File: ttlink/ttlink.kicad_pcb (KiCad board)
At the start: 2 copper layers, 38.6 x 17.9 mm, 10 parts, among them J1 USB, J2 TTL, U1 CH340G, Y1 12MHz

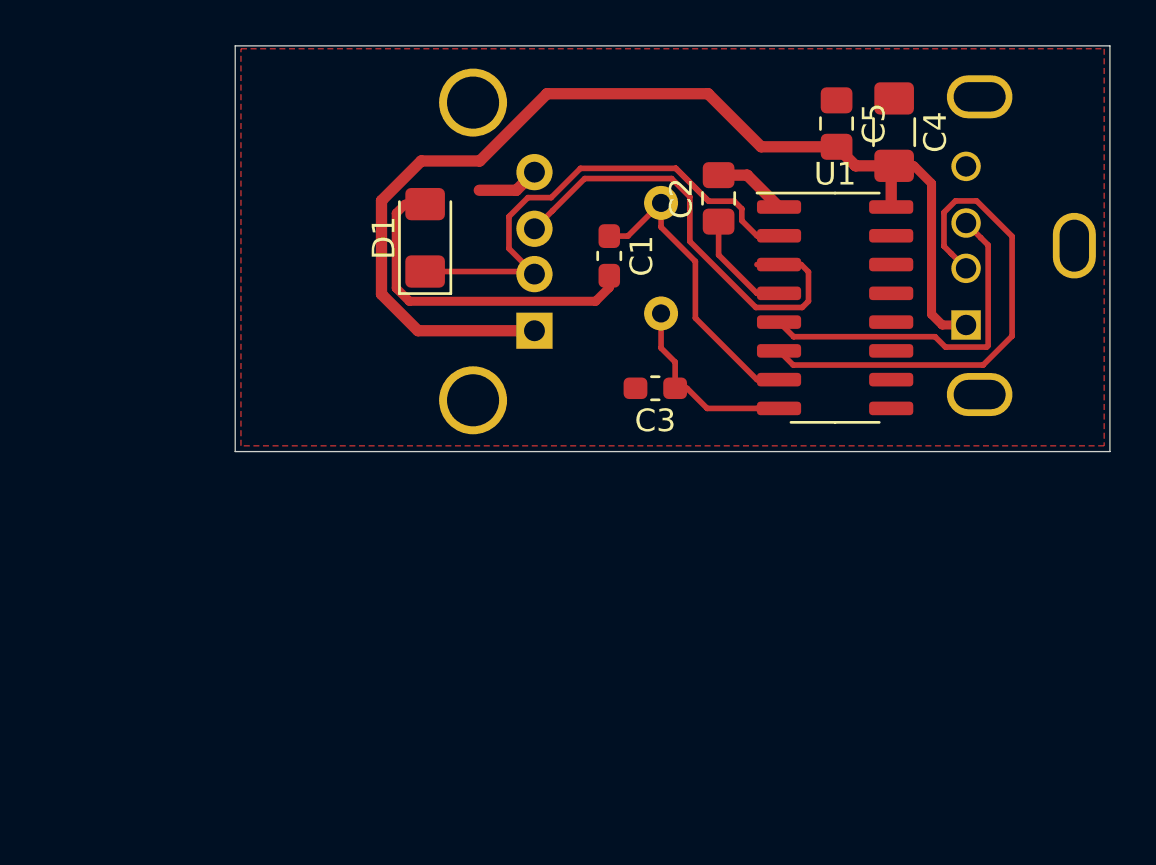
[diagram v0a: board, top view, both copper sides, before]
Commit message: PCB layed out
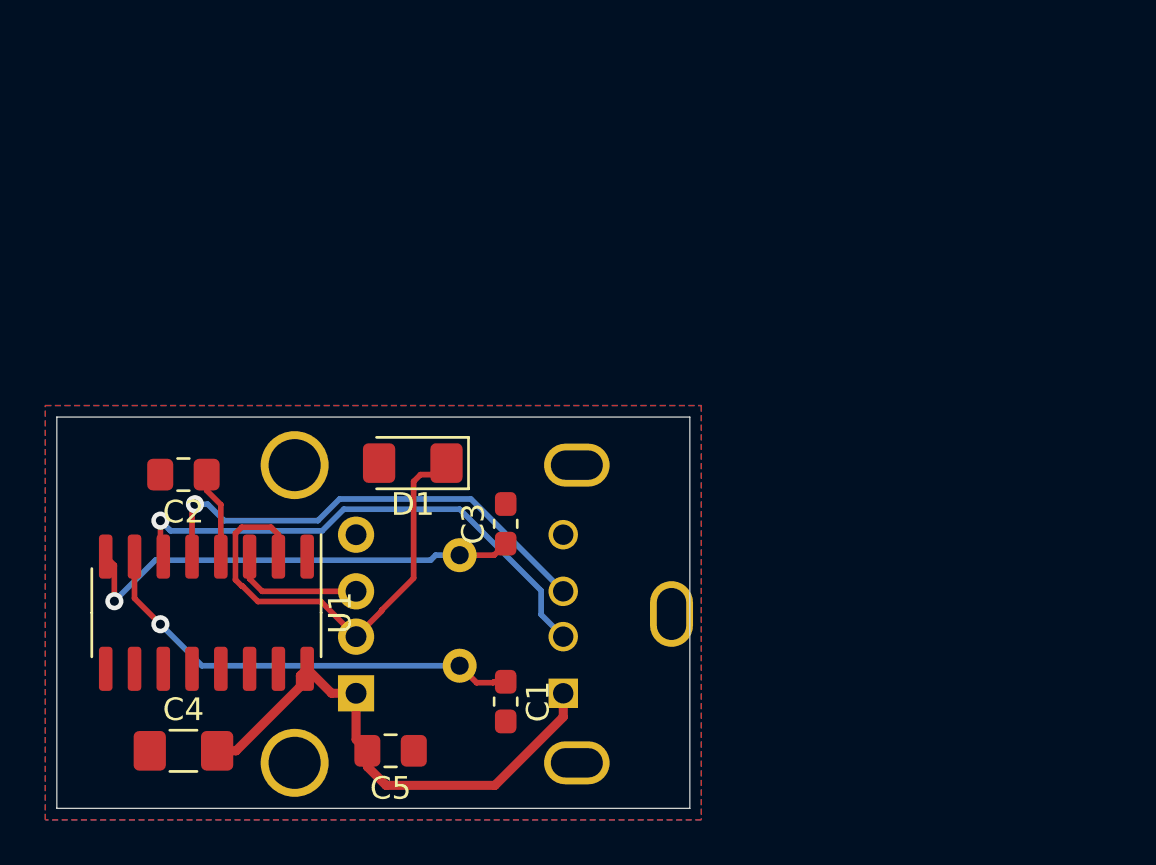
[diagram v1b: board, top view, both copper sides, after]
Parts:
- moved C4 41.6 mm to (100.1, 122.4), turned to 0 degrees
- moved C5 34.0 mm to (109.2, 122.4), turned to 180 degrees
- moved U1 30.8 mm to (101.1, 116.3), turned to 270 degrees
- moved C2 26.6 mm to (100.1, 110.2), turned to 180 degrees
- moved J1 24.1 mm to (116.8, 119.9)
- moved C1 20.2 mm to (114.3, 120.3)
- moved J2 17.8 mm to (107.7, 119.9)
- moved Y1 13.9 mm to (112.3, 113.8), turned to 270 degrees
- moved D1 9.96 mm to (110.2, 109.7), turned to 180 degrees
- moved C3 8.91 mm to (114.3, 112.4), turned to 90 degrees
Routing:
- net +5V: track 48.8 -> 23.1 mm
- net Earth: track 21.2 -> 0.00 mm
- net Net-(J2-Pad3): track 20.3 -> 5.90 mm
- net Net-(C3-Pad1): track 8.51 -> 20.4 mm, vias 0 -> 1
- net Net-(C1-Pad1): track 13.4 -> 20.8 mm, vias 0 -> 1
- net Net-(J1-Pad3): track 15.5 -> 21.7 mm, vias 0 -> 1
- net Net-(D1-Pad1): track 24.3 -> 20.6 mm
- net Net-(C2-Pad1): track 4.84 -> 3.88 mm
- net Net-(J1-Pad2): track 22.2 -> 23.0 mm, vias 0 -> 1
- added copper zone on B.Cu, net Earth
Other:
- board size 38.6 x 17.9 mm -> 27.9 x 17.3 mm
